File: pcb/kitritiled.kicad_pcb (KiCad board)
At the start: 2 copper layers, 22.8 x 22.8 mm, 15 parts, among them J1 ICSP, J2 ICSP, Q1 AO3401A, Q2 AO3400A, SW1 RESET, U1 PIC12LF1571-I/SN, U2 74LVC1G123

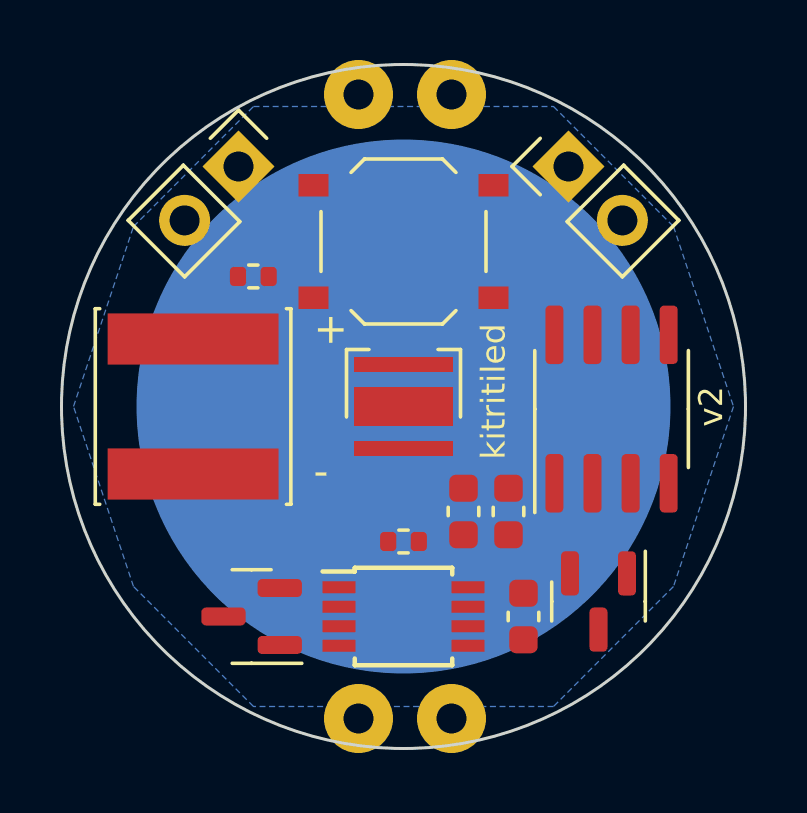
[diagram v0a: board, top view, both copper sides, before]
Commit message: attiny version
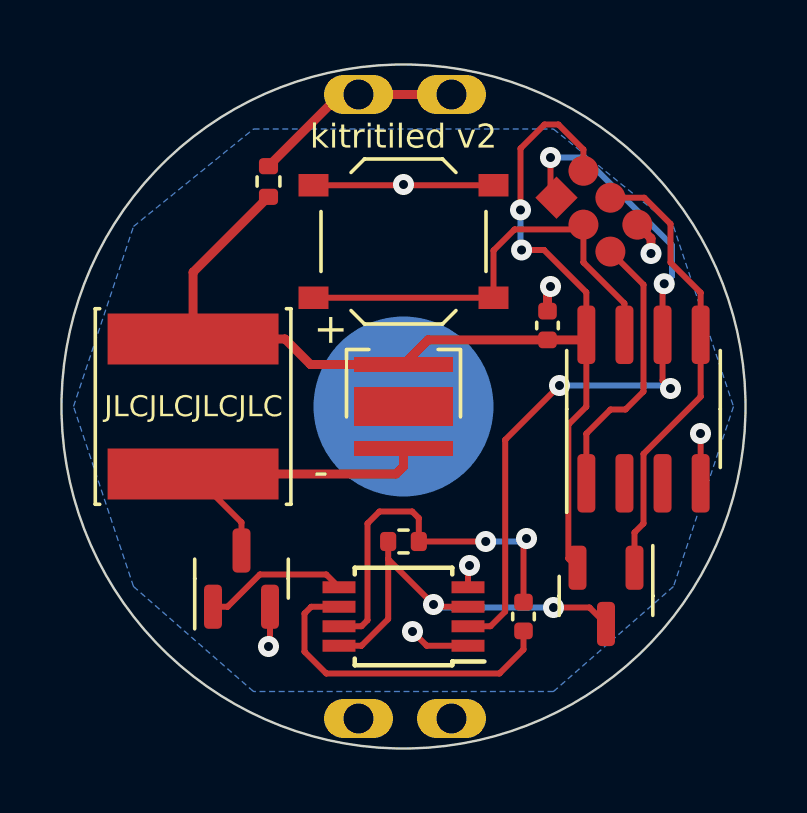
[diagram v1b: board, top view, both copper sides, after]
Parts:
- removed C1: 10u, Capacitor_SMD:C_0603_1608Metric
- removed J1, J2: ICSP, Connector_PinHeader_2.54mm:PinHeader_1x02_P2.54mm_Vertical
- added J4: AVR-ISP-6, Connector_PinHeader_1.27mm:PinHeader_2x03_P1.27mm_Vertical, F.Cu at (95.1, 83.0)
- C2: value 0.1u -> 4u7; footprint Capacitor_SMD:C_0603_1608Metric -> Capacitor_SMD:C_0402_1005Metric
- C3: footprint Capacitor_SMD:C_0603_1608Metric -> Capacitor_SMD:C_0402_1005Metric
- R2: value 59K -> 1K
- U1: value PIC12LF1571-I/SN -> ATtiny13A-SS
- moved C2 6.33 mm to (94.8, 87.3)
- moved R1 3.21 mm to (85.5, 82.5), turned to 90 degrees
- moved Q2 1.31 mm to (84.6, 95.7), turned to 90 degrees
- moved U1 1.06 mm to (98.0, 90.1)
- moved Q1 0.31 mm to (96.8, 96.3)
- turned U2 to 180 degrees
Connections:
- Q1 pad 1: Net-(Q1-G) -> /MOSI
- SW1 pad 1: Net-(SW1-A) -> /SCK
- U1 pad 1: +3V0 -> /RST
- U1 pad 2: Net-(Q1-G) -> unconnected-(U1-PB3-Pad2)
- U1 pad 3: Net-(U1-RA4) -> unconnected-(U1-PB4-Pad3)
- U1 pad 4: Net-(SW1-A) -> GND
- U1 pad 5: unconnected-(U1-RA2-Pad5) -> /MOSI
- U1 pad 6: ICSP_CLK -> /MISO
- U1 pad 7: ICSP_DATA -> /SCK
- U1 pad 8: GND -> +3V0
- U2 pad 2: Net-(U1-RA4) -> /MISO
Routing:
- net +3V0: track 0.00 -> 38.8 mm, vias 0 -> 2
- net /MISO: track 0.00 -> 25.2 mm, vias 0 -> 4
- net /SCK: track 0.00 -> 15.2 mm
- net /MOSI: track 0.00 -> 15.2 mm
- net CLR: track 0.00 -> 13.9 mm, vias 0 -> 2
- net GND: track 0.00 -> 13.8 mm, vias 0 -> 7
- net Net-(U2A-RCext): track 0.00 -> 12.8 mm, vias 0 -> 2
- net Net-(U2A-Cext): track 0.00 -> 11.1 mm
- net Net-(D1-A): track 0.00 -> 10.9 mm
- net /RST: track 0.00 -> 9.26 mm
- net Net-(BT1-+): track 0.00 -> 7.09 mm
- net Net-(Q2-G): track 0.00 -> 4.82 mm
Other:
- board text added: "JLCJLCJLCJLC"
- board text added: "kitritiled v2"
- board text removed: "3V"
- board text removed: "CLK"
- board text removed: "DATA"
- board text removed: "GND"
- board text removed: "kitritiled"
- board text removed: "v2"
